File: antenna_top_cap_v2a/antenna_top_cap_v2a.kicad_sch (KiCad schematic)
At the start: 32 parts, among them J1 DEBUG, J12 USB_C_Receptacle_USB2.0_16P, J2 Battery Charge Bypass, J3 FC Reset Jumper, J4 FC USB Bootselect Jumper, J5 Conn_Coaxial, Q1 BSS138, U1 VL6180XV0NR/1, U16 MCP9808T-E/MS, U2 LP5907-2.8V, U3 NCS1.5-232+, U4 VEML7700

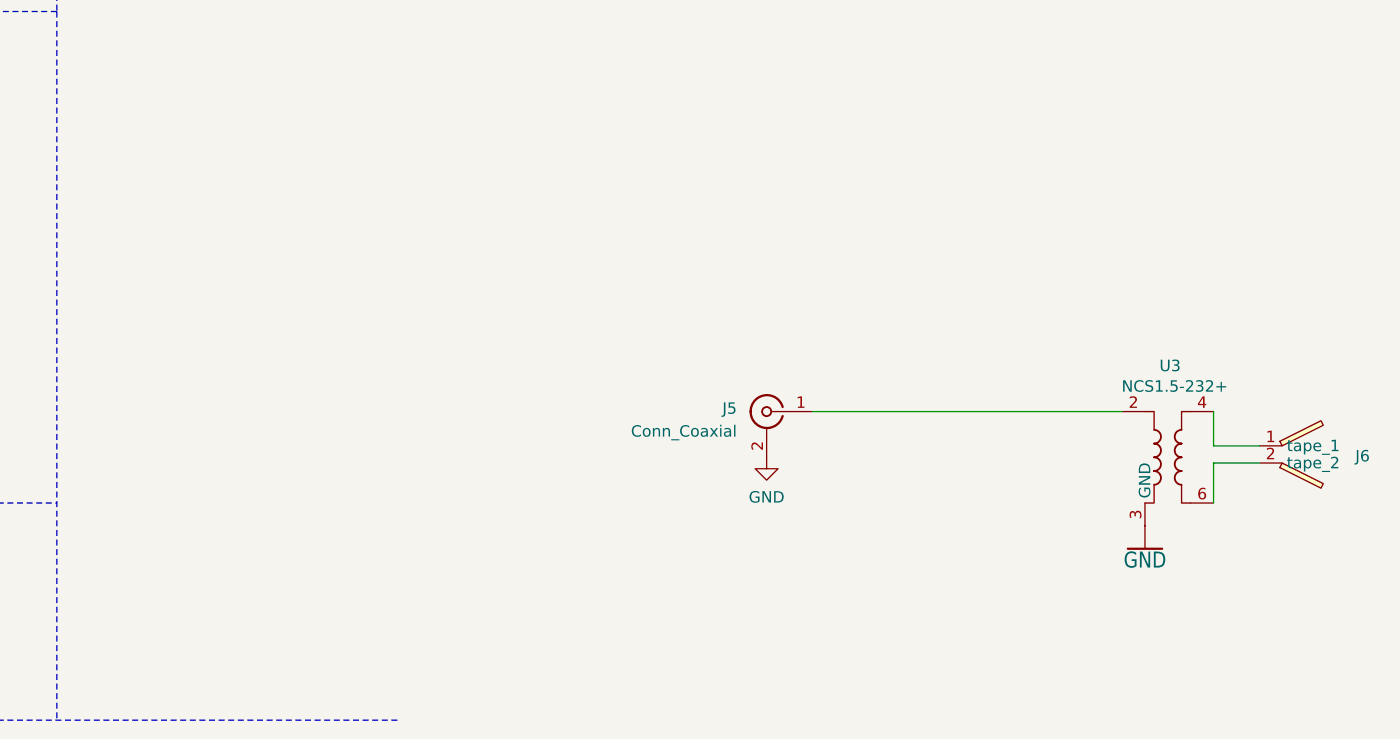
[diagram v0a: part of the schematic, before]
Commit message: Production Files as Ordered 4/17/2025
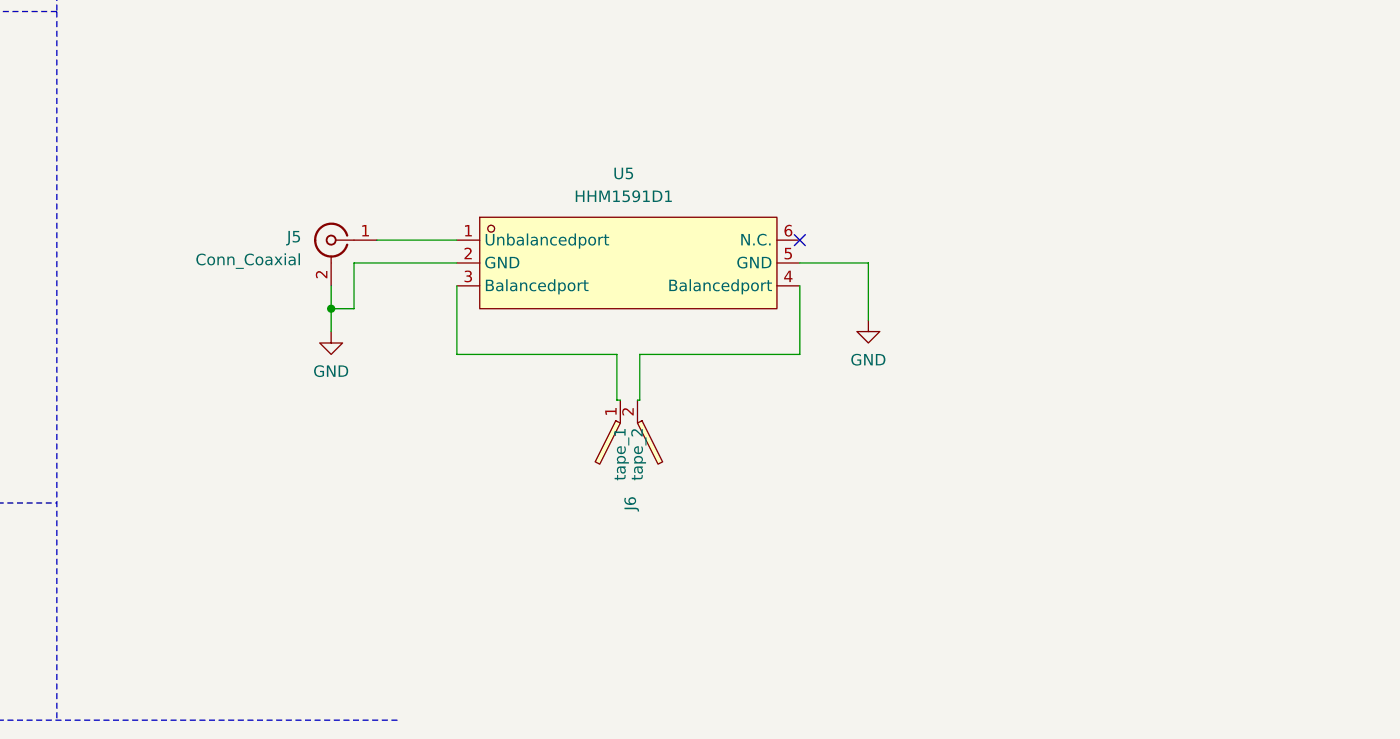
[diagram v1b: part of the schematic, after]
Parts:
- removed U3: NCS1.5-232+, RF_Converter:Balun_Johanson_0896BM15A0001, symbol Transformer:0433BM15A0001
- added U5: HHM1591D1, easyeda2kicad:XFMR-SMD_HHM1591D1, symbol easyeda2kicad:HHM1591D1
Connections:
- net GND: now also U5.2 (GND), U5.5 (GND)
- net at J6.1 (tape_1): now also U5.3 (Balancedport)
- net at J6.2 (tape_2): now also U5.4 (Balancedport)
- net at J5.1 (In): now also U5.1 (Unbalancedport)
- no-connect marks 12 -> 13
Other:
- moved on the sheet: J5, J6
